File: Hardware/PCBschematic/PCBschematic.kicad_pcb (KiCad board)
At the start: 2 copper layers, 69.5 x 50.9 mm, 49 parts, among them J3 Conn_01x02, J4 Conn_02x07_Odd_Even, J5 Conn_01x02, J6 Conn_01x02, J7 Conn_01x02, J8 batterie, J9 Conn_01x08, Q1 SQ2310ES, Q2 SQ2310ES, Q3 SQ2310ES, Q4 SQ2310ES, SW1 SW_Push, SW2 SW_Push, U1 STM32L412KBTx, U2 NCS210, U3 NCS210, U4 NCS210, U5 NCS210, U6 regulator_17395xx36

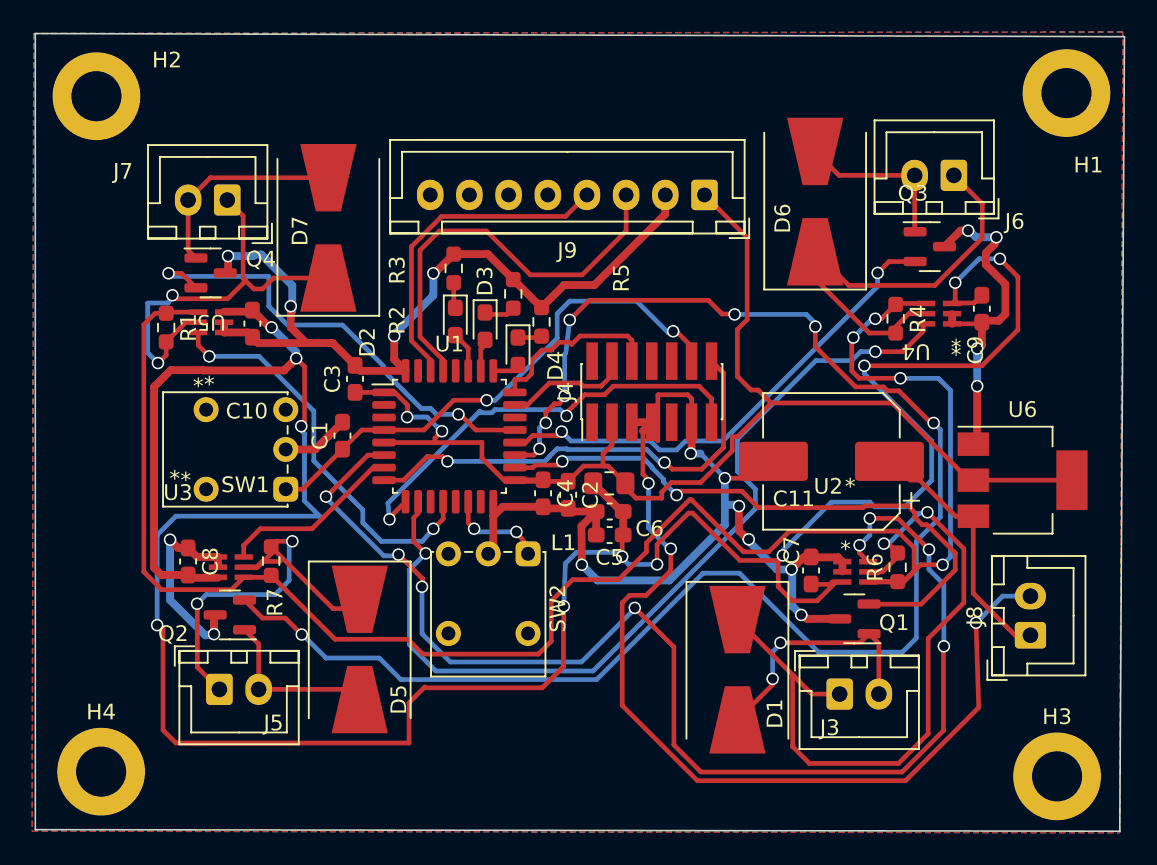
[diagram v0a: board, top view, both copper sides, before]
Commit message: routage v1
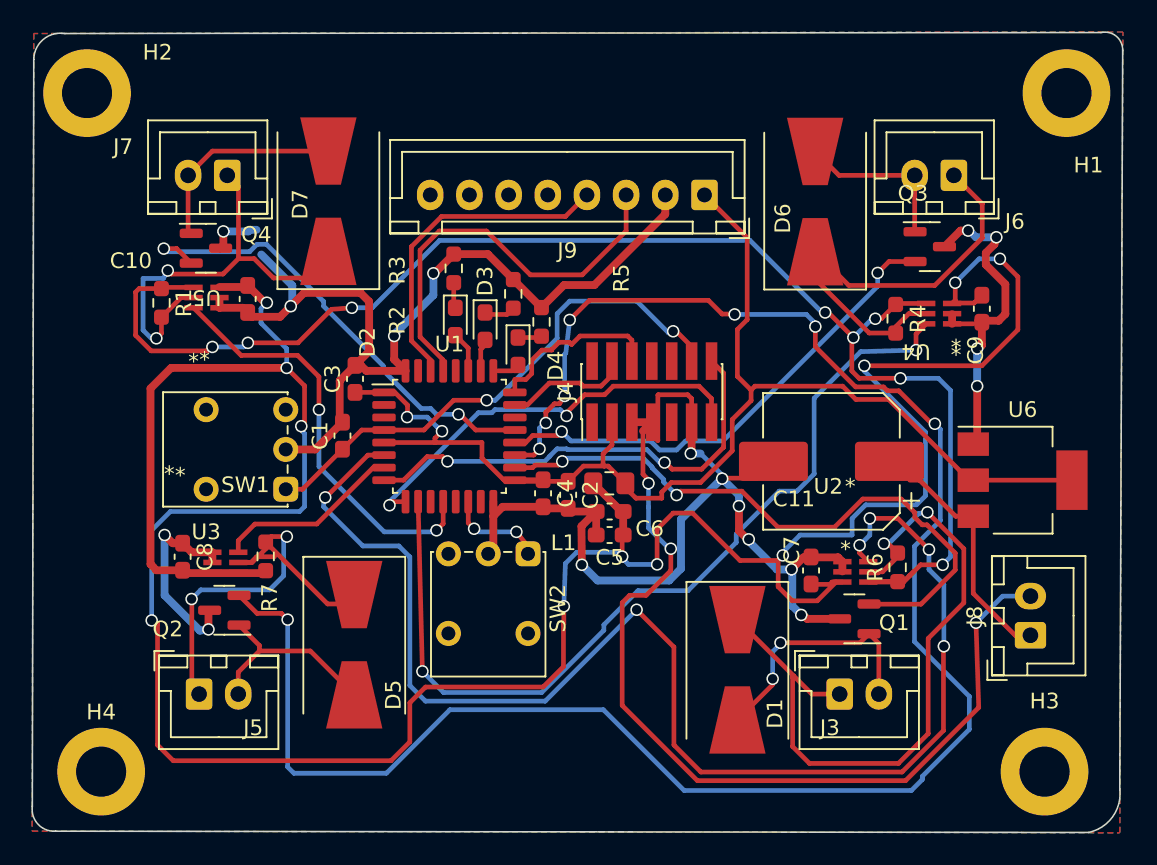
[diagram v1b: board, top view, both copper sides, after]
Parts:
- moved D7 1.70 mm to (142.1, 102.2)
- moved C10 1.60 mm to (136.9, 108.4)
- moved Q4 1.60 mm to (134.3, 105.2)
- moved R1 1.60 mm to (131.4, 108.7)
- moved U5 1.60 mm to (134.3, 108.3)
- moved J7 1.58 mm to (135.7, 100.5)
- moved J5 1.33 mm to (133.8, 133.7)
- moved H3 1.28 mm to (187.8, 137.9)
- moved H2 0.78 mm to (126.7, 95.0)
- moved D5 0.46 mm to (143.8, 130.5)
- moved C8 0.46 mm to (132.8, 124.9)
- moved Q2 0.46 mm to (135.5, 128.3)
- moved R7 0.46 mm to (138.1, 124.9)
- moved U3 0.46 mm to (135.5, 125.2)
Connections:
- R7 pad 1: VCC -> +3.3VA
- U3 pad 4: VCC -> +3.3VA
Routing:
- net VCC: track 115.4 -> 92.8 mm, vias 4 -> 8
- net PWM_2: track 104.2 -> 123.7 mm
- net GND: track 212.4 -> 220.7 mm
- net +3.3VA: track 178.3 -> 185.3 mm
- net AO1: track 81.4 -> 86.6 mm, vias 8 -> 6
- net USART2_RX: track 28.7 -> 27.2 mm
- net PWM_1: track 39.2 -> 40.6 mm
- net AO4: track 25.7 -> 27.1 mm
- net Net-(D5-A): track 11.3 -> 12.7 mm
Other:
- board size 69.5 x 50.9 mm -> 69.6 x 51.1 mm
